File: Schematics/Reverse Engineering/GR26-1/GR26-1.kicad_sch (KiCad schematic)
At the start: 135 parts, among them J1 Conn_01x40

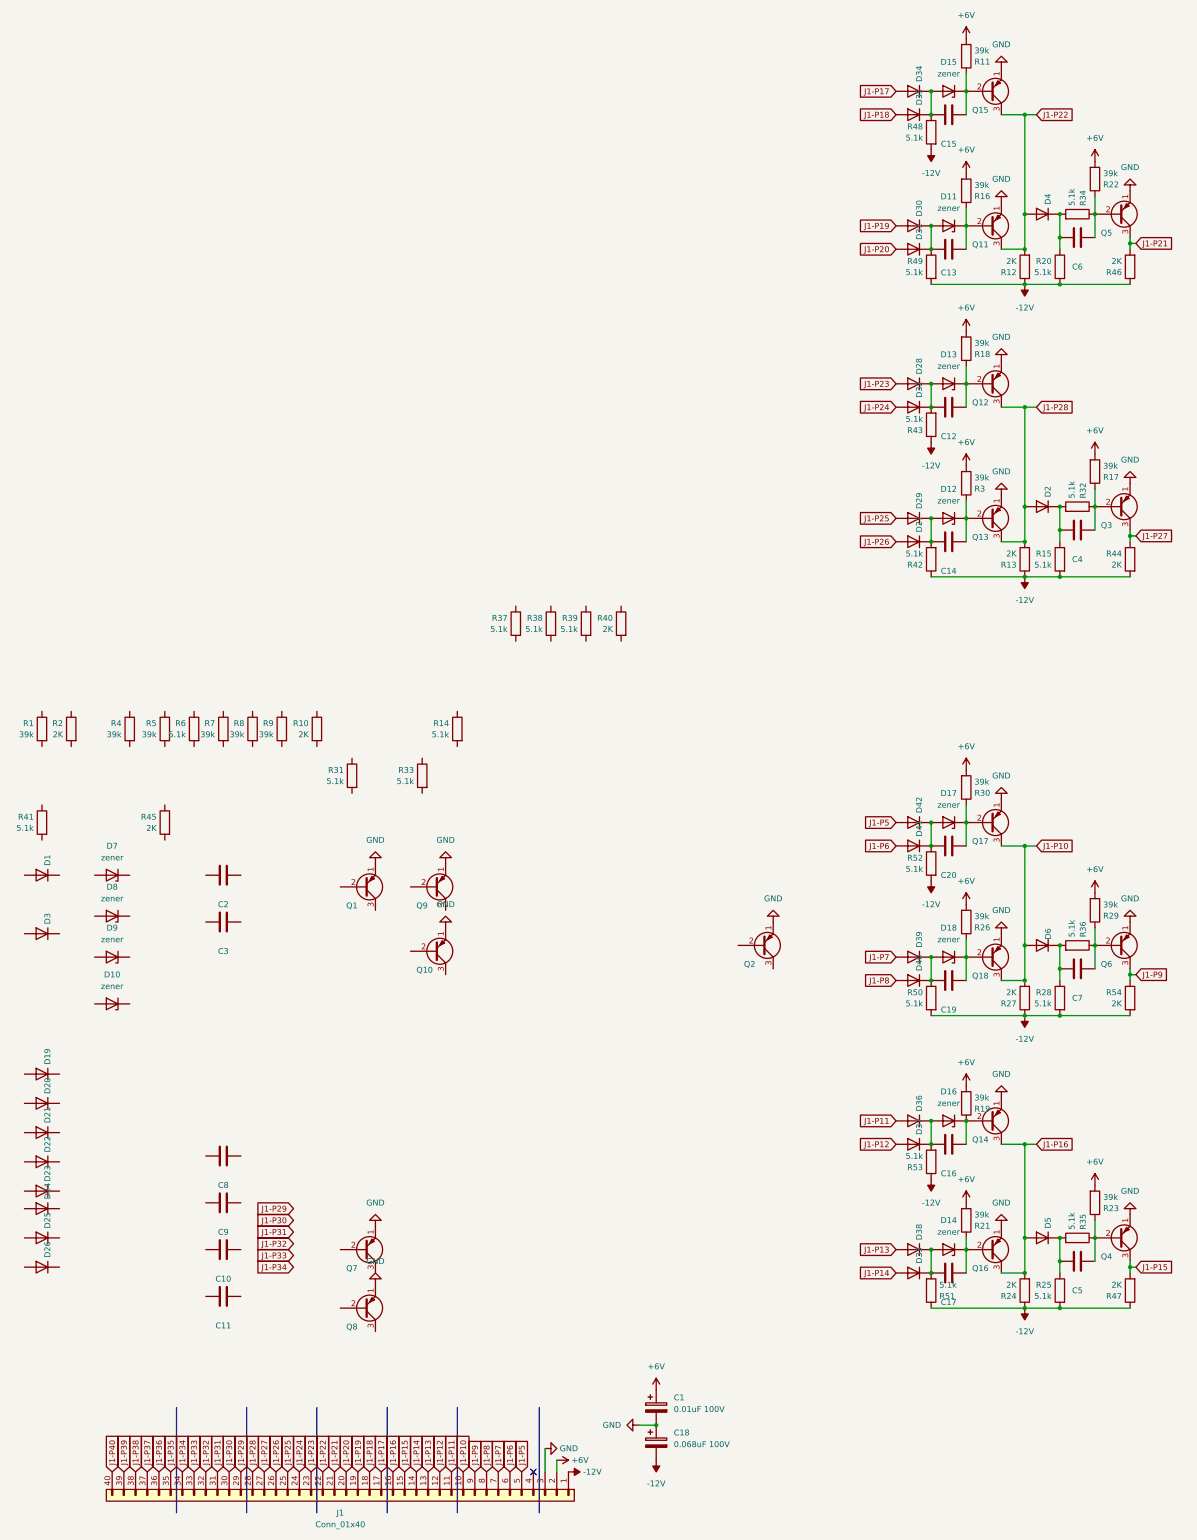
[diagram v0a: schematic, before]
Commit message: Completed GR26-1
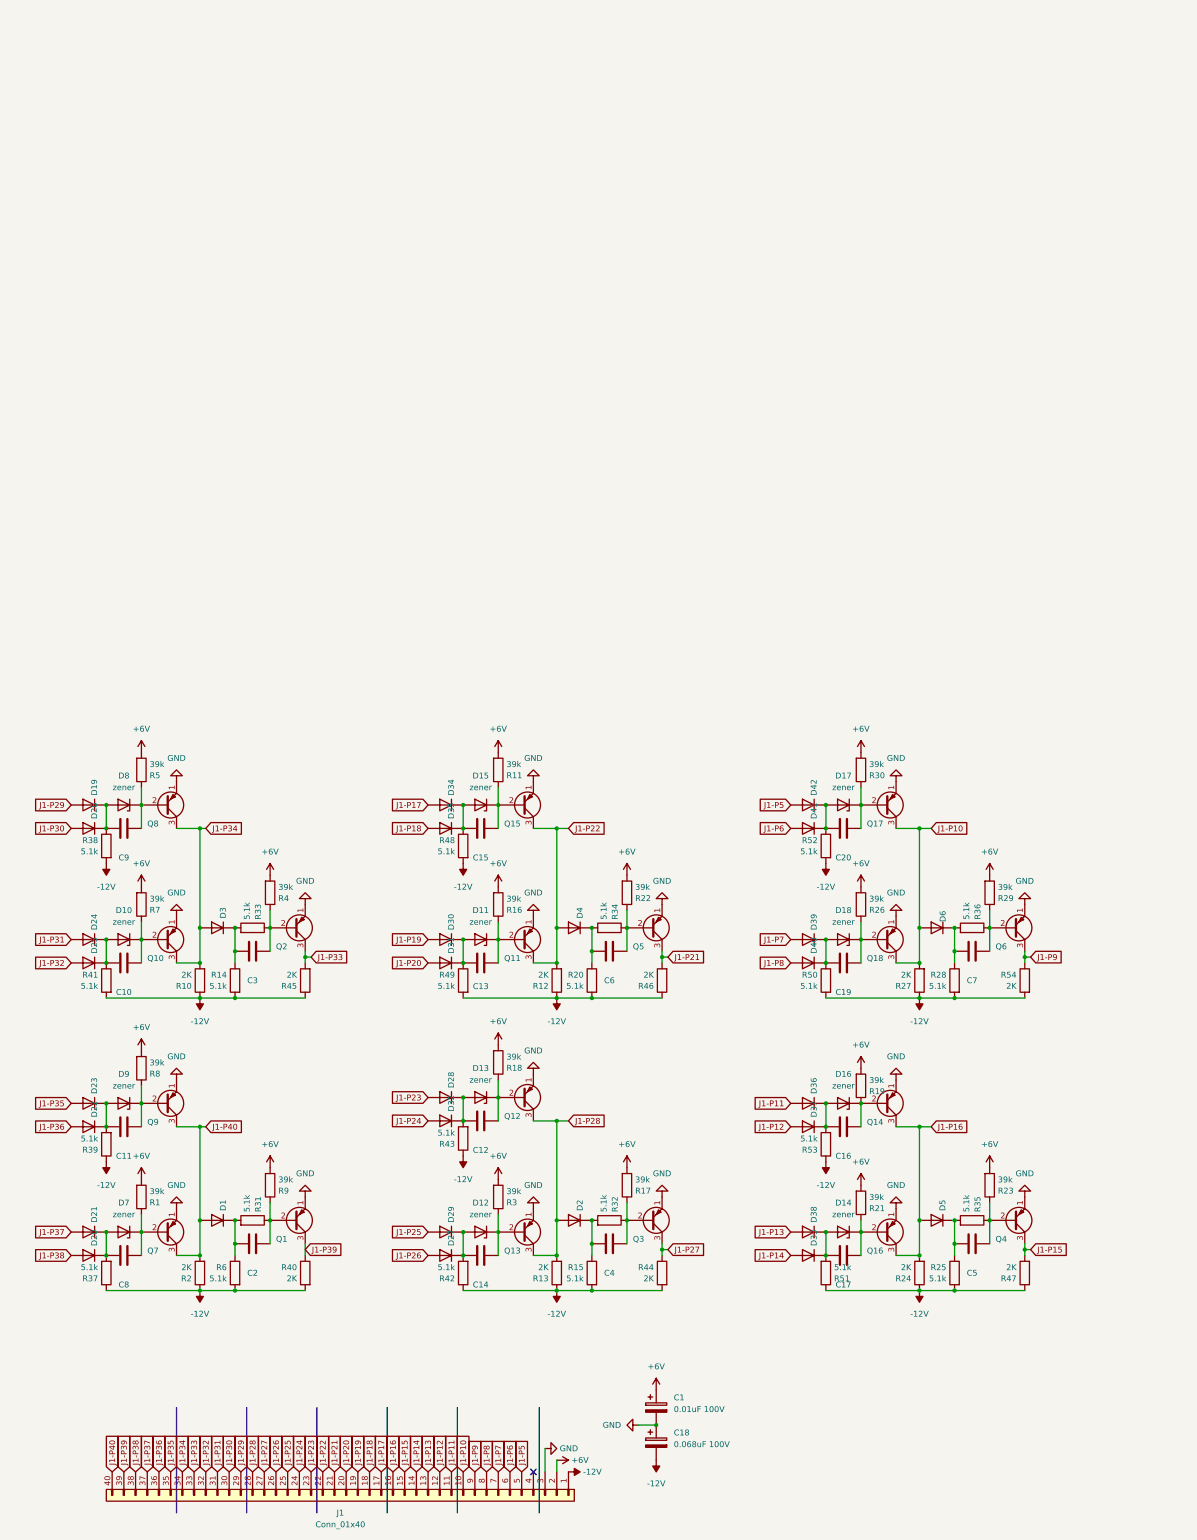
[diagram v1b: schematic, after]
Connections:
- net +6V: now also R1.2, R4.2, R5.2, R7.2, R8.2, R9.2
- net -12V: now also R10.1, R14.2, R2.1, R37.1, R38.2, R39.1, R40.2, R41.2, R45.1, R6.2
- net J1-P29: now also D19.2 (A)
- net J1-P30: now also D26.2 (A)
- net J1-P31: now also D24.2 (A)
- net J1-P32: now also D25.2 (A)
- net J1-P33: now also Q2.3 (C), R45.2
- net J1-P34: now also D3.2 (A), Q10.3 (C), Q8.3 (C), R10.2
- net J1-P35: now also D23.2 (A)
- net J1-P36: now also D22.2 (A)
- net J1-P37: now also D21.2 (A)
- net J1-P38: now also D20.2 (A)
- net J1-P39: now also Q1.3 (C), R40.1
- net J1-P40: now also D1.2 (A), Q7.3 (C), Q9.3 (C), R2.2
- net at Q8.2 (B): now also C9.2, D8.1 (K), R5.1
- net at D25.1 (K): now also C10.1, D10.2 (A), D24.1 (K), R41.1
- net at C3.1: now also Q2.2 (B), R33.1, R4.1
- net at C3.2: now also D3.1 (K), R14.1, R33.2
- net at D19.1 (K): now also C9.1, D26.1 (K), D8.2 (A), R38.1
- net at R6.1: now also C2.2, D1.1 (K), R31.2
- net at R31.1: now also C2.1, Q1.2 (B), R9.1
- net at C11.1: now also D22.1 (K), D23.1 (K), D9.2 (A), R39.2
- net at C11.2: now also D9.1 (K), Q9.2 (B), R8.1
- net at R1.1: now also C8.2, D7.1 (K), Q7.2 (B)
- net at R7.1: now also C10.2, D10.1 (K), Q10.2 (B)
- net at R37.2: now also C8.1, D20.1 (K), D21.1 (K), D7.2 (A)
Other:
- moved on the sheet: C10, C11, C12, C13, C14, C15, C16, C17, C19, C2, C20, C3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
